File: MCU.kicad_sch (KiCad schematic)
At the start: 1 part, among them U1 STM32L476RCTx

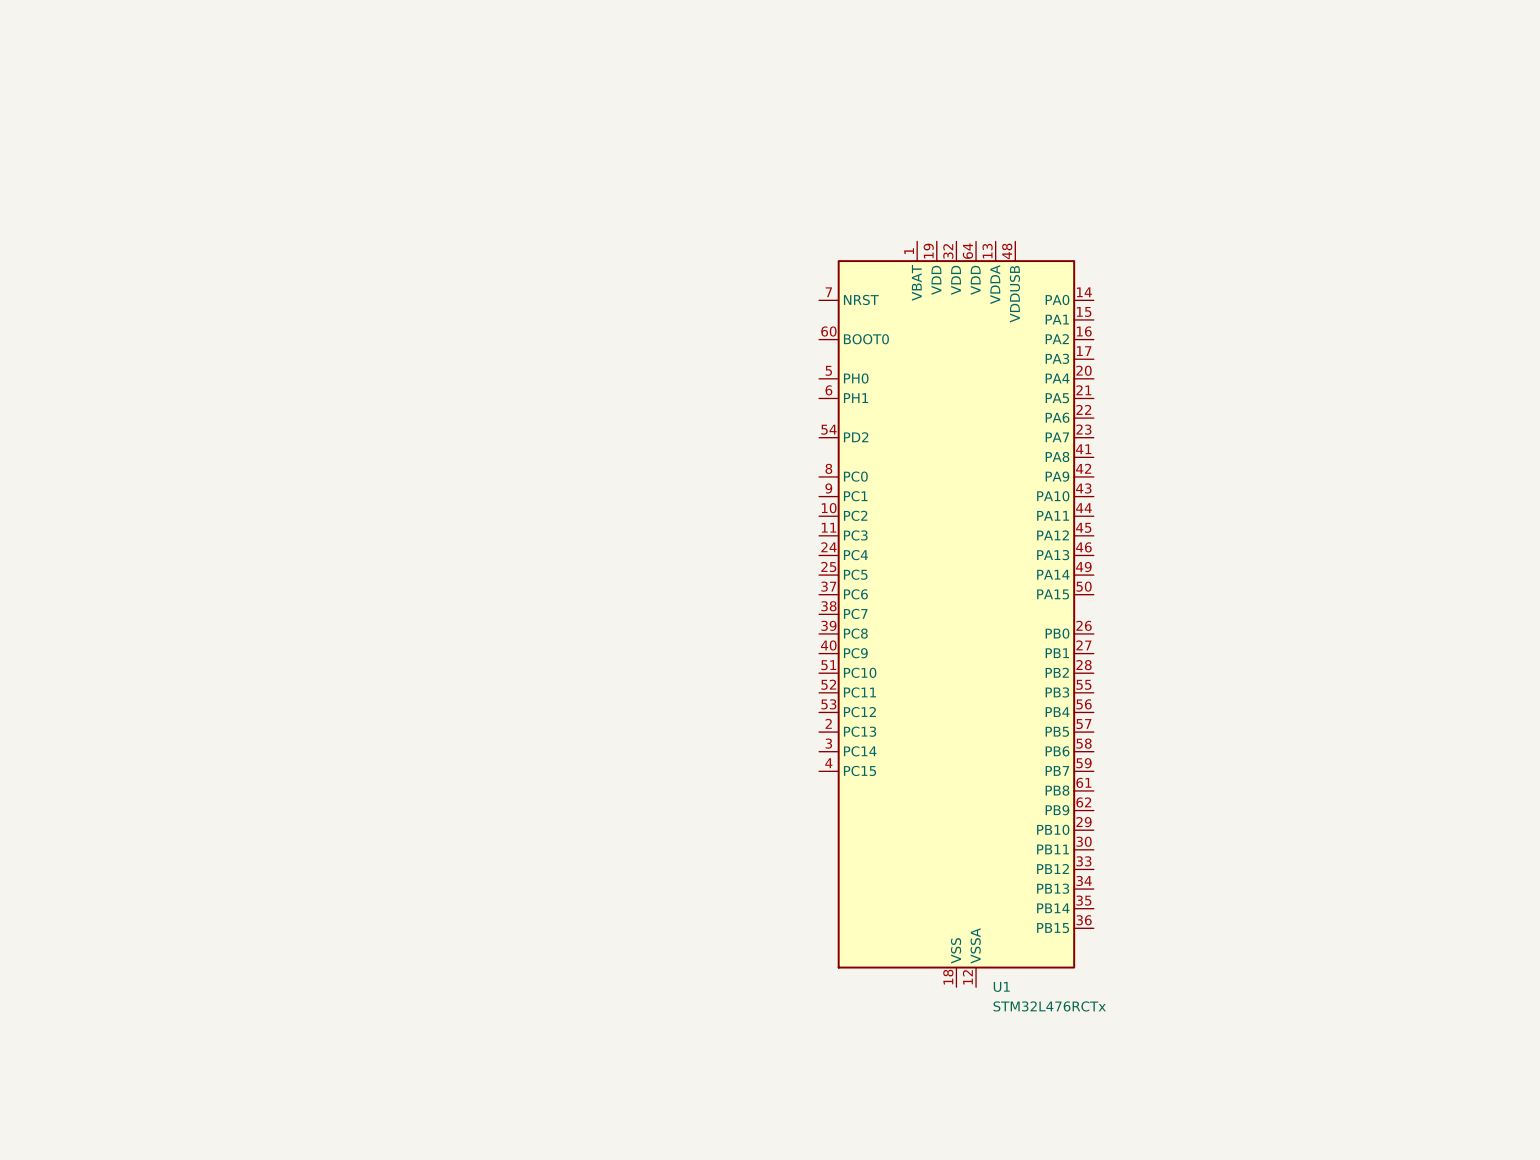
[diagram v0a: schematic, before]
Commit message: This should be the most recent one
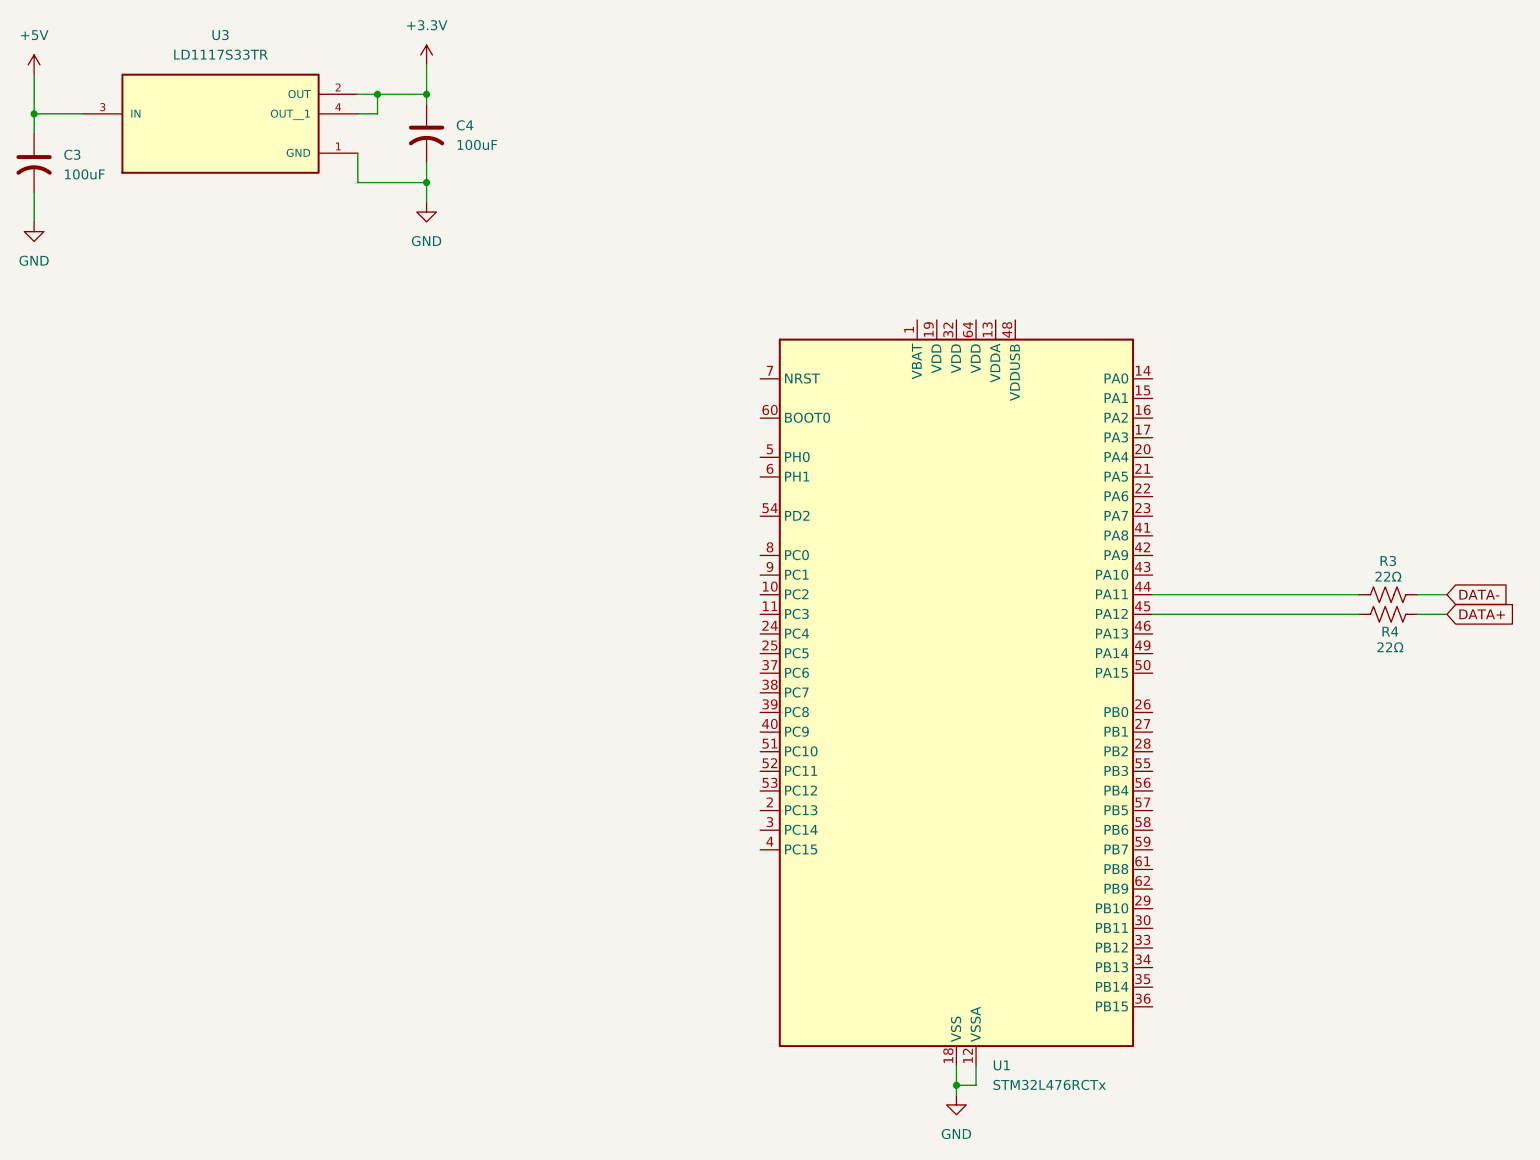
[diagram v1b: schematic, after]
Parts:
- added C3, C4: 100uF, symbol Device:C_US
- added R3, R4: 22Ω, symbol Device:R_US
- added U3: LD1117S33TR, LD1117S33TR:SOT230P700X180-4N, symbol LD1117S33TR:LD1117S33TR
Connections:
- net GND: now reaches U1.12 (VSSA)
- net GND: now also U1.18 (VSS), U1.31 (VSS), U1.47 (VSS), U1.63 (VSS), C3.2, C4.2, U3.1 (GND)
- net at U1.44 (PA11): now also R3.1
- net at U1.45 (PA12): now also R4.1
- new net +3.3V: C4.1, U3.2 (OUT), U3.4 (OUT__1)
- new net +5V: C3.1, U3.3 (IN)
- new net DATA+: R4.2
- new net DATA-: R3.2
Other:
- moved on the sheet: U1
